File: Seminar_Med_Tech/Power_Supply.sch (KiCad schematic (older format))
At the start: 1 part

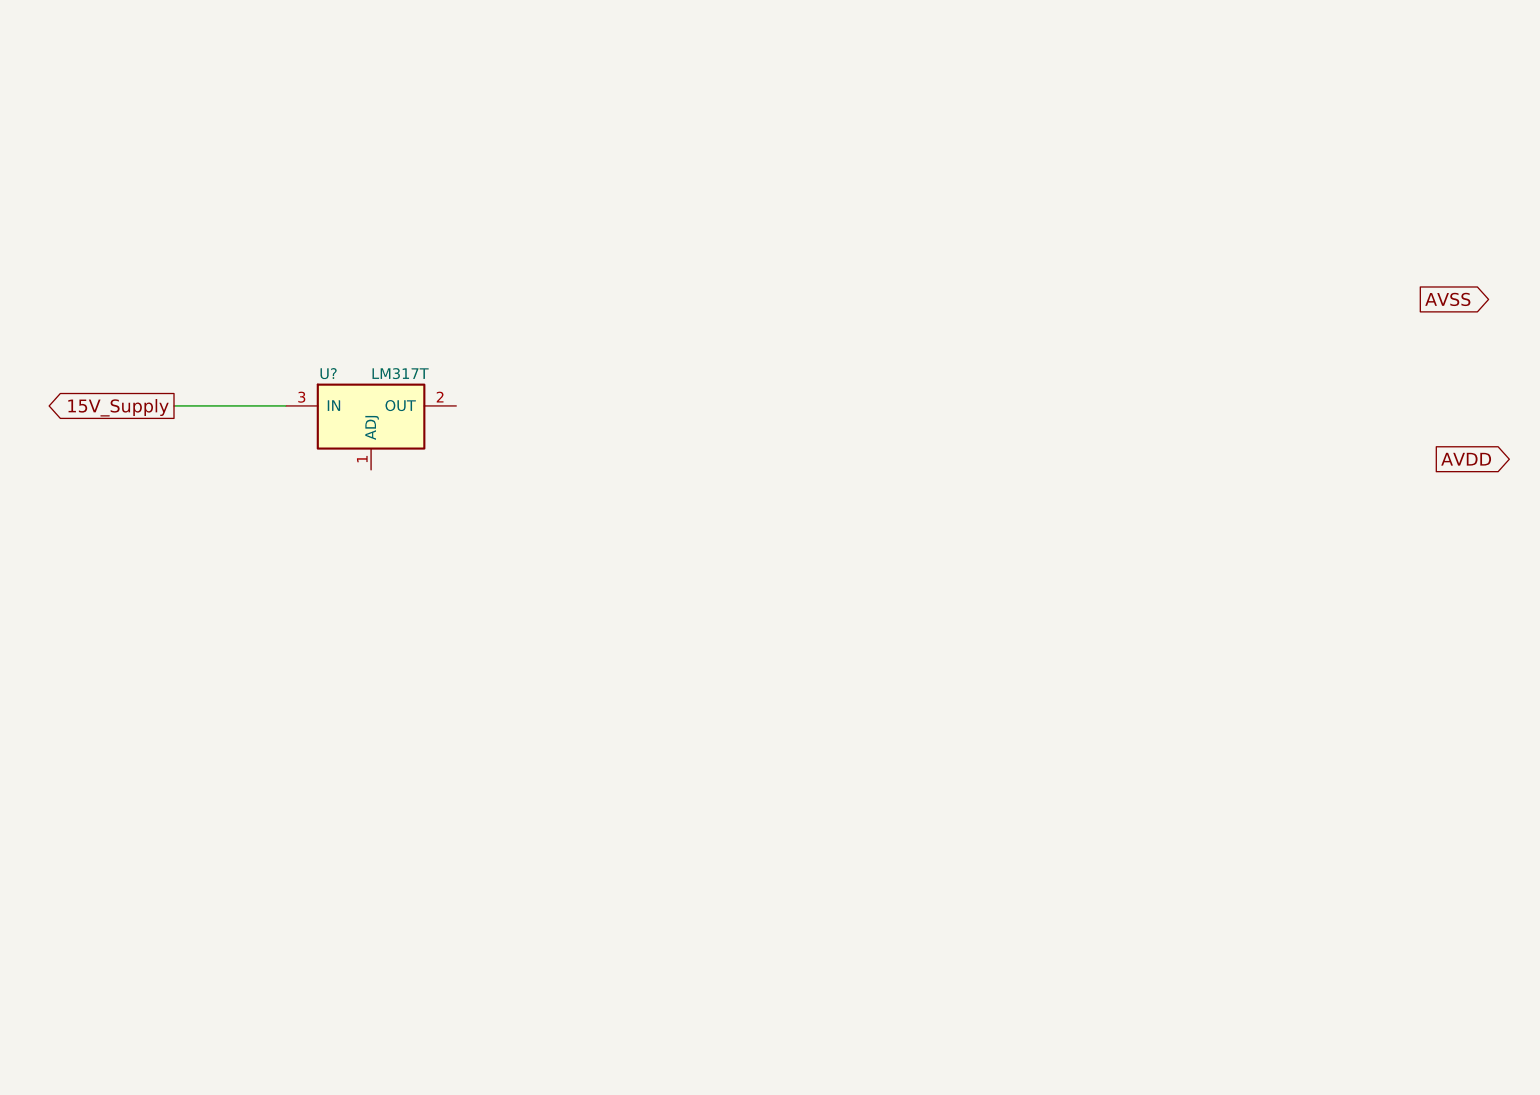
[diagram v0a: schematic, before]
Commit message: Updated
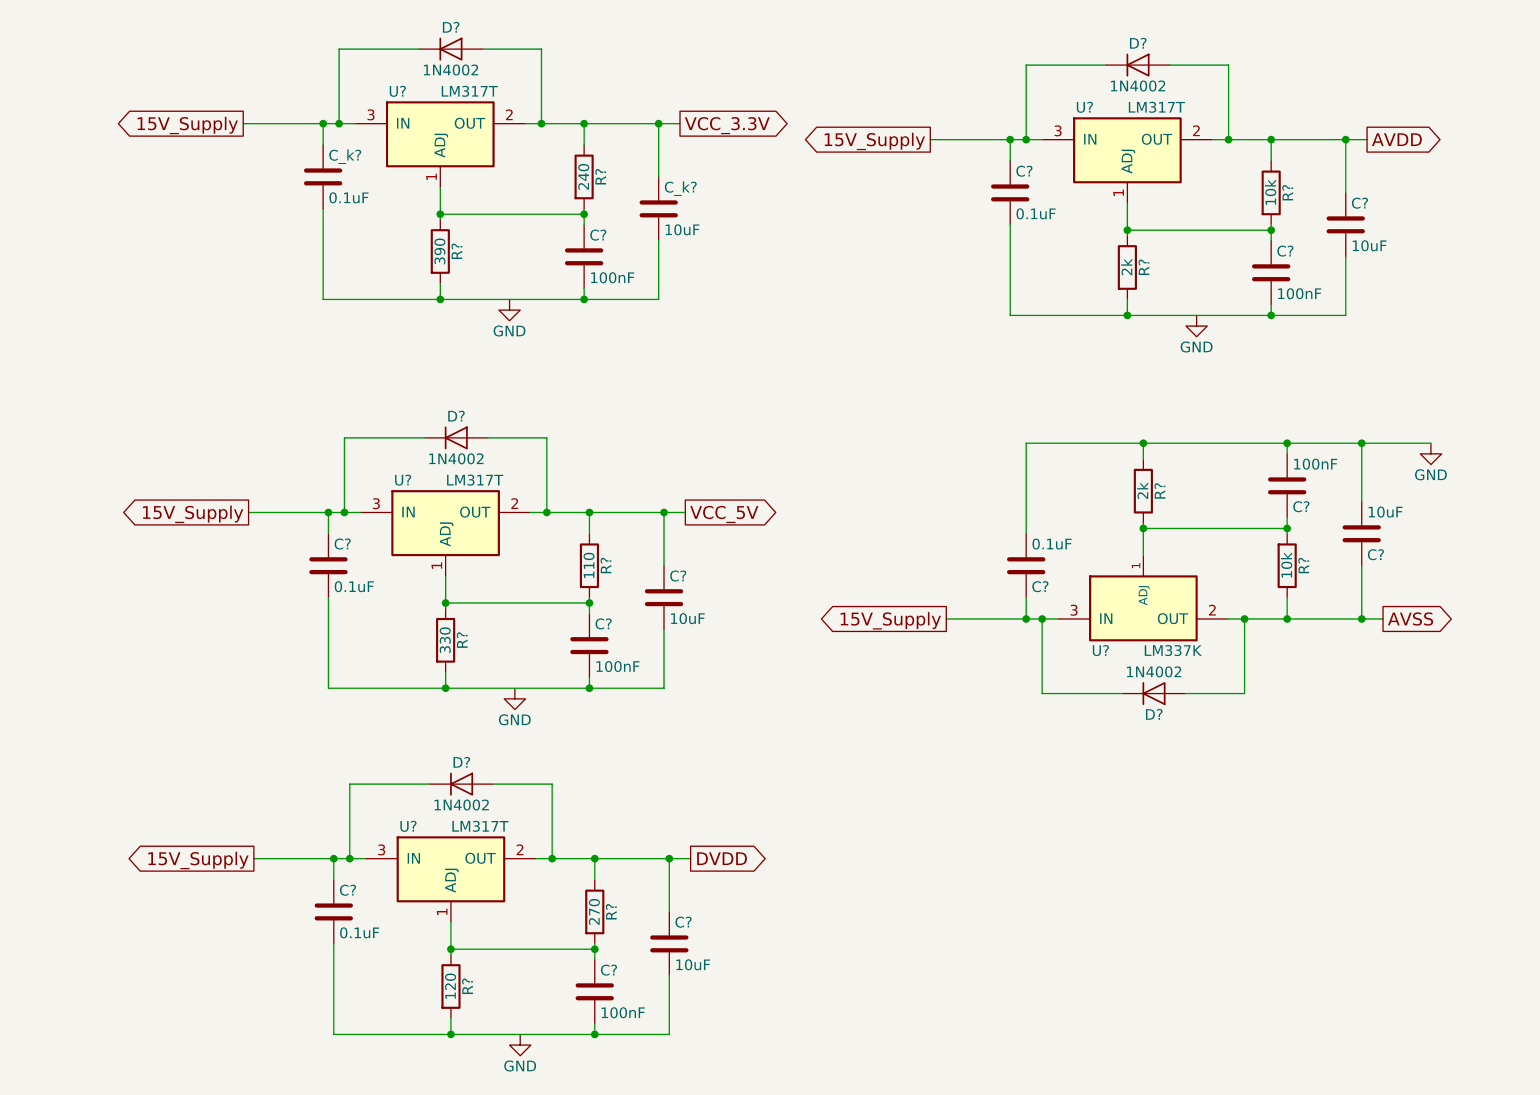
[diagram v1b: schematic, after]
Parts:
- added C? (x5): 100nF, symbol C
- added C? (x4), C_k?: 0.1uF, symbol C
- added C? (x4), C_k?: 10uF, symbol C
- added D? (x5): 1N4002, symbol D
- added R?: 240, symbol R
- added R?: 390, symbol R
- added R?: 110, symbol R
- added R?: 330, symbol R
- added R? (x2): 10k, symbol R
- added R? (x2): 2k, symbol R
- added R?: 270, symbol R
- added R?: 120, symbol R
- added U? (x3): LM317T, TO_SOT_Packages_THT:TO-220_Vertical, symbol LM317T
- added U?: LM337K, TO_SOT_Packages_THT:TO-3, symbol LM337K
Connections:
- net 15V_Supply: now also C?.1, C?.1, C?.1, C?.1, C_k?.1, D?.1 (K), D?.1 (K), D?.1 (K), D?.1 (K), D?.1 (K), U?.3 (IN), U?.3 (IN), U?.3 (IN), U?.3 (IN)
- net AVDD: now also C?.1, D?.2 (A), R?.1, U?.2 (OUT)
- net AVSS: now also C?.1, D?.2 (A), R?.1, U?.2 (OUT)
- net at U?.1 (ADJ): now also C?.1, R?.1, R?.2
- net VCC_3.3V: now reaches U?.2 (OUT)
- net VCC_3.3V: now also C_k?.1, D?.2 (A), R?.1
- new net: C?.2, C_k?.2, C_k?.2, R?.2
- new net: C?.1, R?.1, R?.2, U?.1 (ADJ) (x4)
- new net: C?.2, C?.2, C?.2, R?.2 (x3)
- new net DVDD: C?.1, D?.2 (A), R?.1, U?.2 (OUT)
- new net GND: C?.2, C?.2, C?.2, R?.2
- new net VCC_5V: C?.1, D?.2 (A), R?.1, U?.2 (OUT)
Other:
- moved on the sheet: U?
